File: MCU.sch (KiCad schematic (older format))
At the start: 8 parts, among them P2 MCU_JTAG, U12 DA28F320J5-120, U13 MC68340PV16E, U15 MAX6314, U16 74HCT138D, U6 IDT7024S25PF, U8 KM681000CLG-7L, U9 KM681000CLG-7L

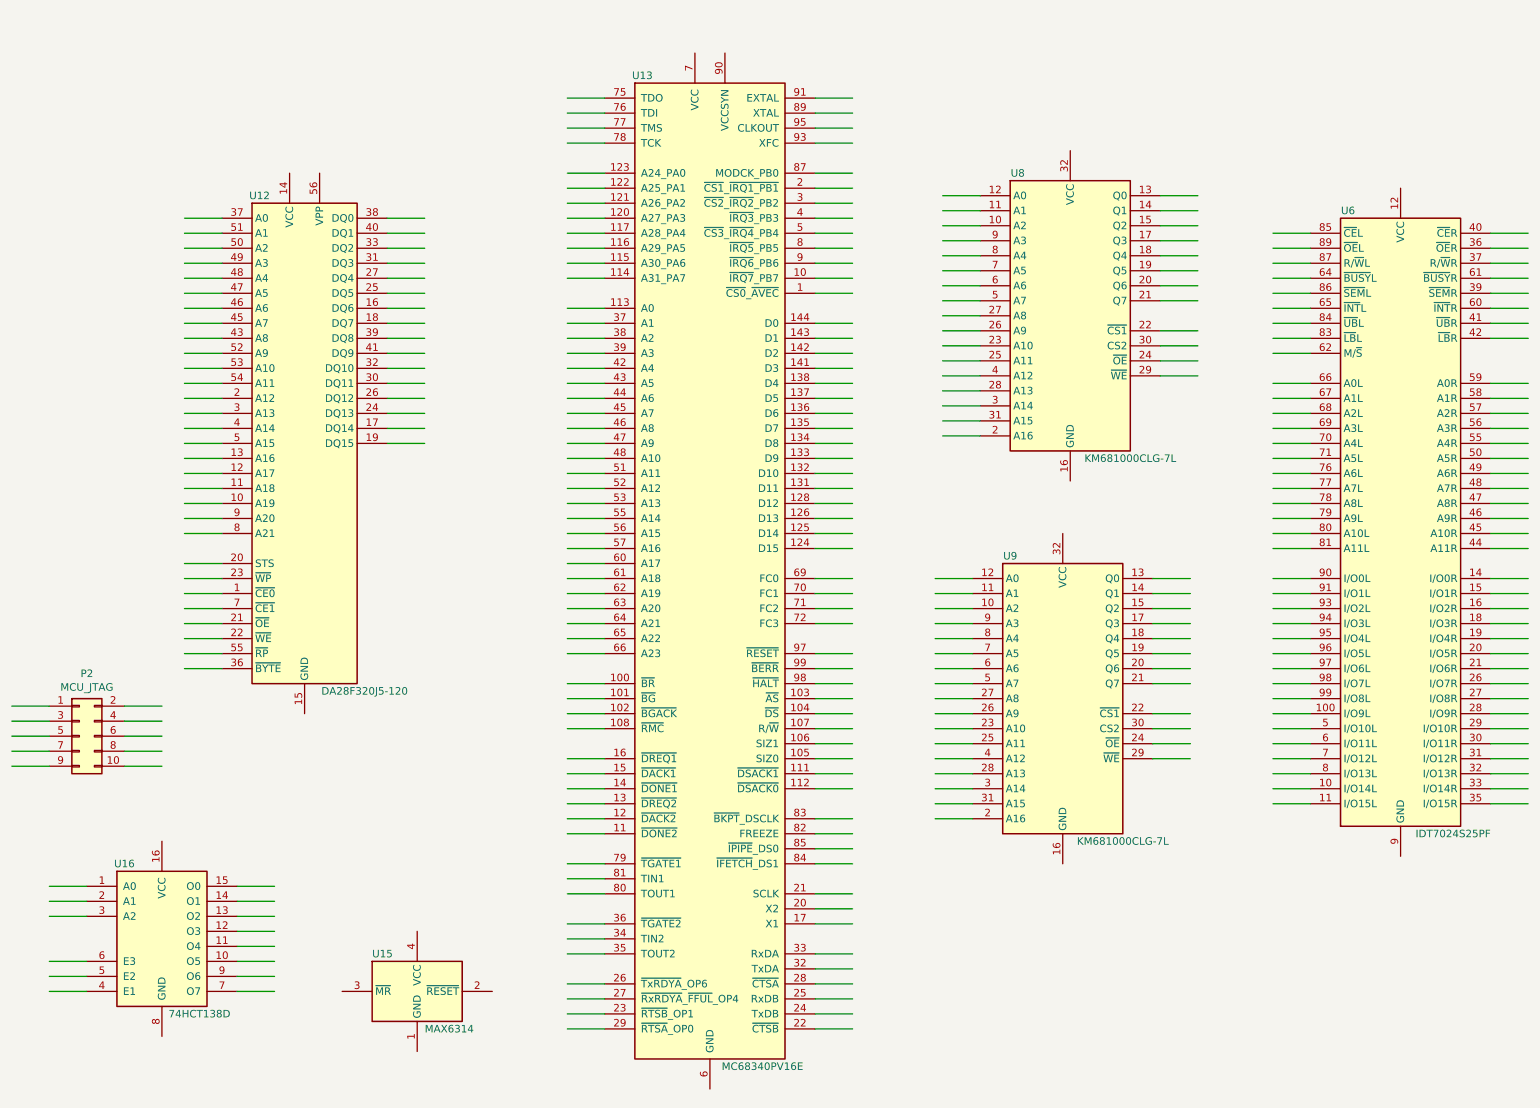
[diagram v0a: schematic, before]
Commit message: MCU start
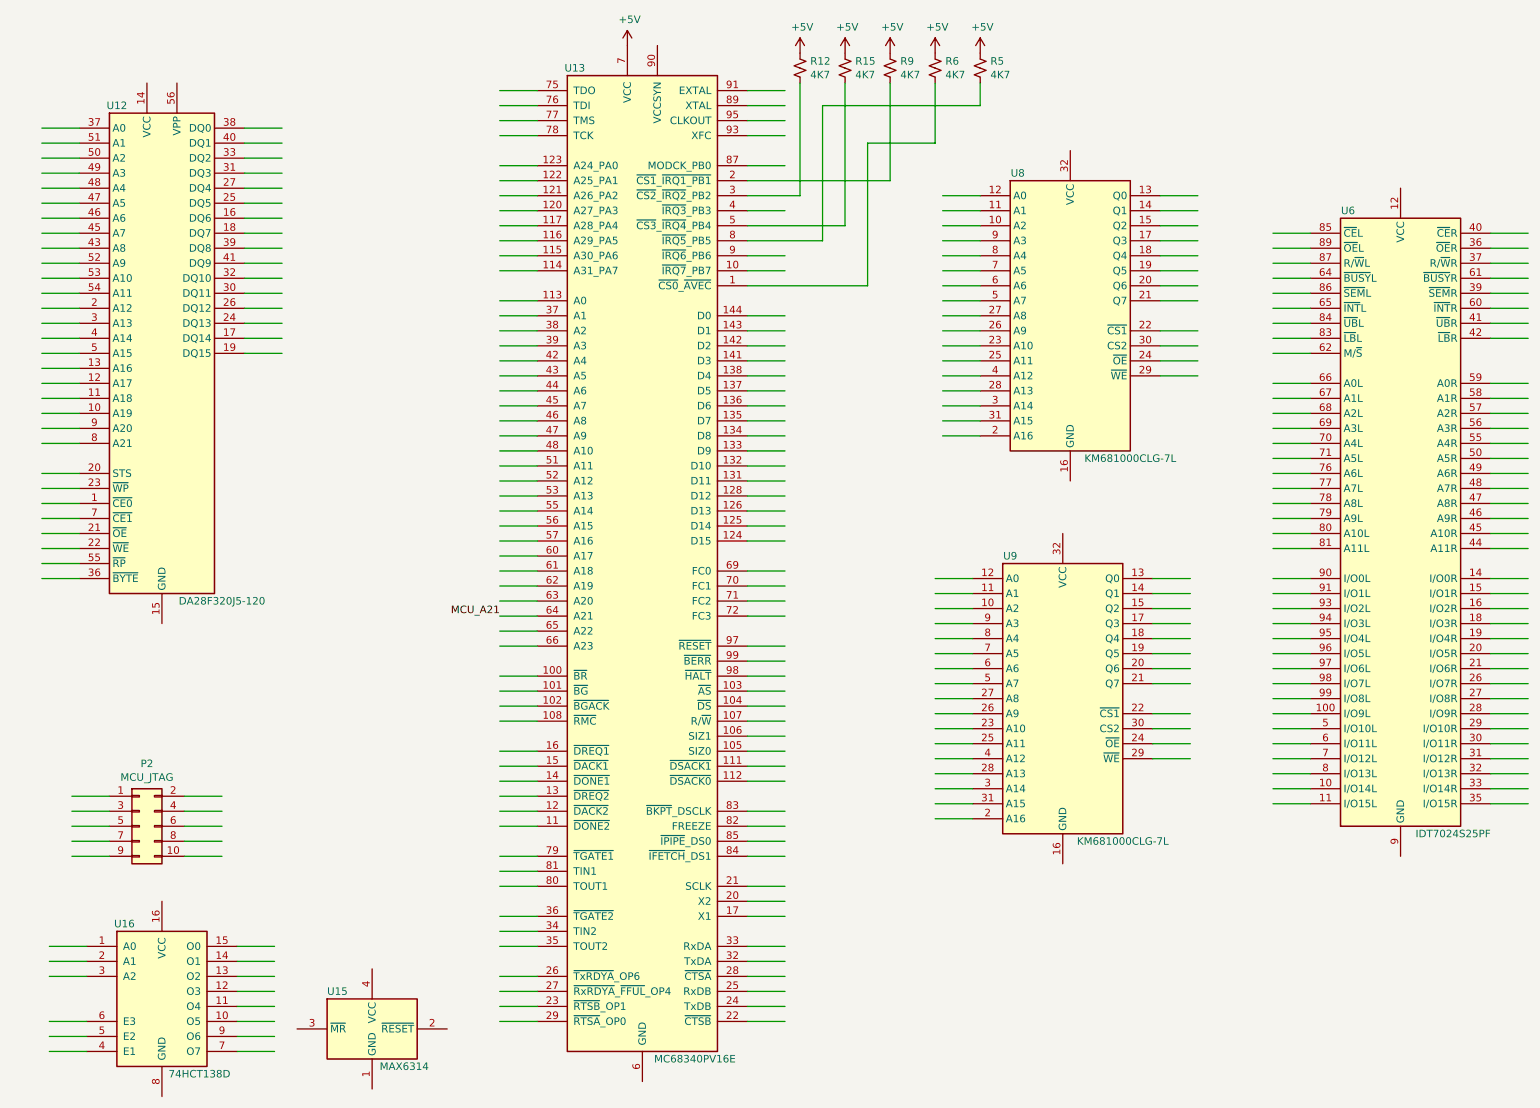
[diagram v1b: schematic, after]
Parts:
- added R12, R15, R5, R6, R9: 4K7, symbol N64DEV:R_Small_US
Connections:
- net labels added: +5V, MCU_A21
- wire segments 313 -> 322
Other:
- moved on the sheet: P2, U12, U13, U15, U16
